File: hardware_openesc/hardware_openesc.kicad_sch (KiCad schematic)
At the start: 0 parts

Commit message: images
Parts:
- added C1, C2: 1u, symbol Device:C_Small
- added Q1, Q2, Q3, Q4, Q5, Q6: BSC007N04LS6, easyeda2kicad:PG-TDSON-8-FL_L5.0-W6.0-P1.27-LS6.2-BL, symbol easyeda2kicad:BSC007N04LS6
- added U1: EFM8BB21F16G-C-QFN20, easyeda2kicad:QFN-20_L3.0-W3.0-P0.50-BL-EP1.7_EFM8BB21F16G, symbol easyeda2kicad:EFM8BB21F16G-C-QFN20
- added U2: FD6288Q_C328453, easyeda2kicad:QFN-24_L4.0-W4.0-P0.50-BL-EP2.6, symbol easyeda2kicad:FD6288Q_C328453
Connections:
- new net: C1.2, C2.2, U1.4 (VDD)
- new net: Q6.1 (S), Q6.2 (S), Q6.3 (S)
- new net: Q5.1 (S), Q5.2 (S), Q5.3 (S), Q6.5 (D), Q6.6 (D), Q6.7 (D), Q6.8 (D)
- new net: Q5.5 (D), Q5.6 (D), Q5.7 (D), Q5.8 (D)
- new net: Q3.1 (S), Q3.2 (S), Q3.3 (S), Q4.5 (D), Q4.6 (D), Q4.7 (D), Q4.8 (D)
- new net: Q3.5 (D), Q3.6 (D), Q3.7 (D), Q3.8 (D)
- new net: Q2.1 (S), Q2.2 (S), Q2.3 (S)
- new net: Q1.1 (S), Q1.2 (S), Q1.3 (S), Q2.5 (D), Q2.6 (D), Q2.7 (D), Q2.8 (D)
- new net: Q4.1 (S), Q4.2 (S), Q4.3 (S)
- new net: Q1.5 (D), Q1.6 (D), Q1.7 (D), Q1.8 (D)
- new net GND: C1.1, C2.1, U1.12 (GND), U1.21 (GND), U1.3 (GND)
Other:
- note added: "A"
- note added: "B"
- note added: "C"

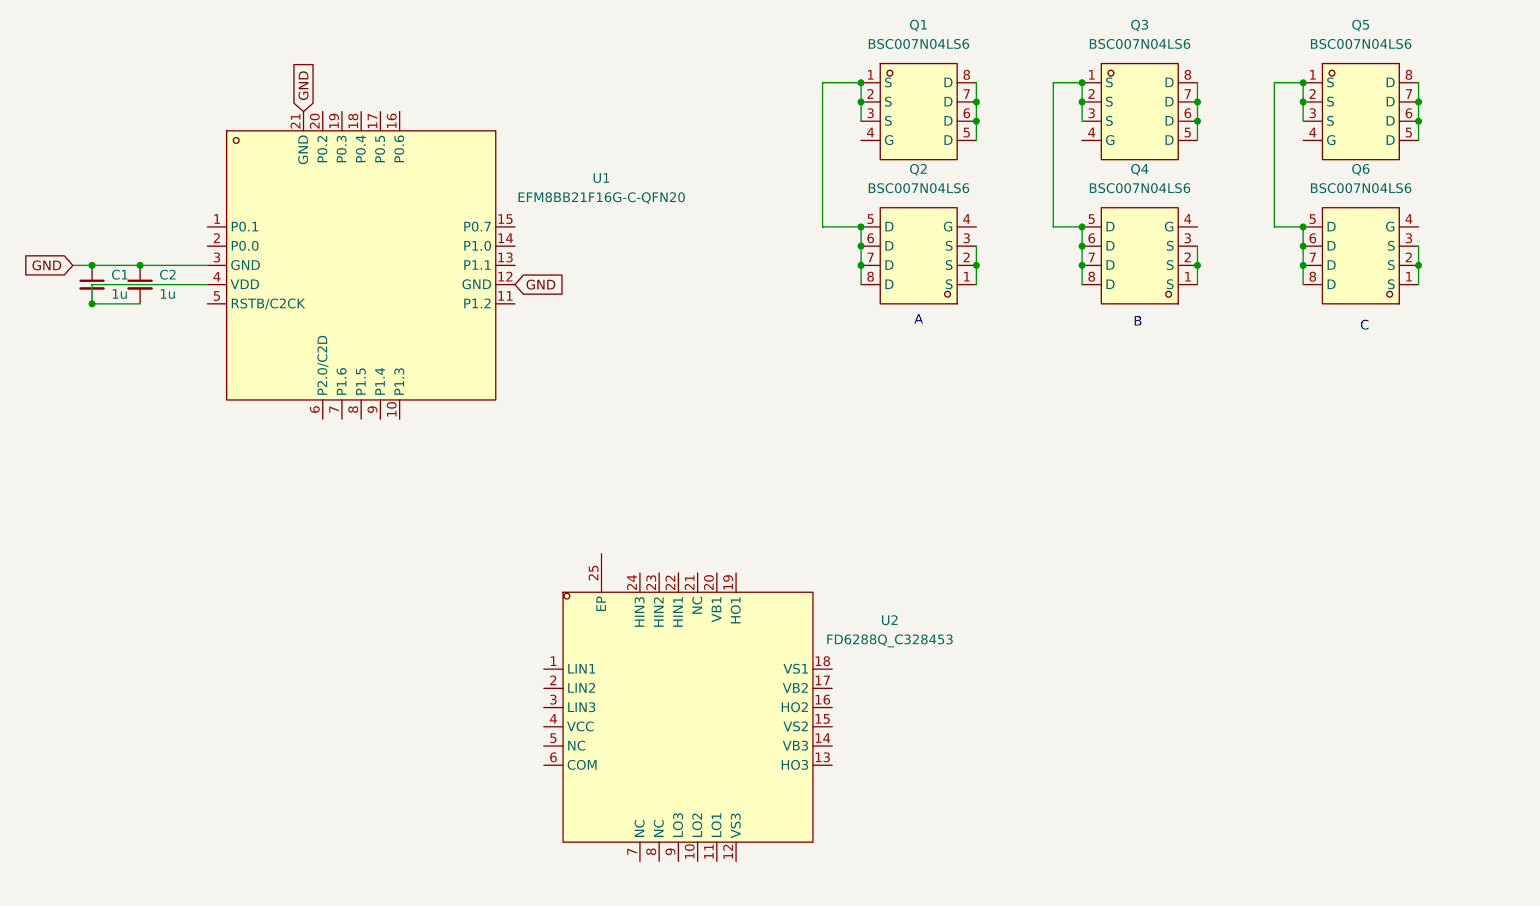
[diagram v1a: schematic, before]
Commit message: schematic
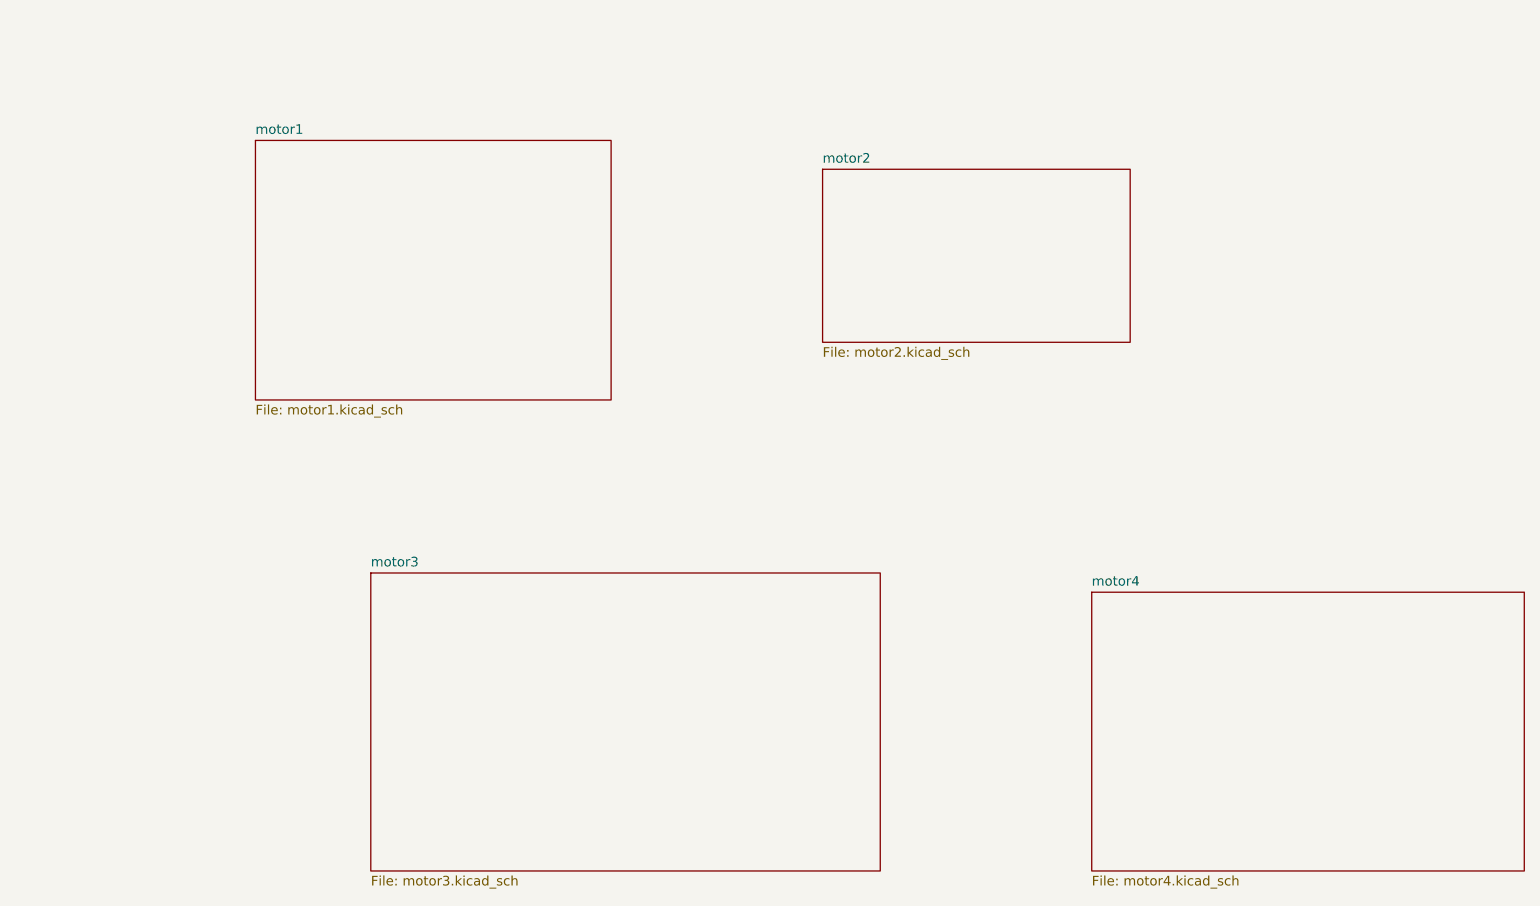
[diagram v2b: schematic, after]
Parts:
- removed C1, C2: 1u, symbol Device:C_Small
- removed Q1, Q2, Q3, Q4, Q5, Q6: BSC007N04LS6, easyeda2kicad:PG-TDSON-8-FL_L5.0-W6.0-P1.27-LS6.2-BL, symbol easyeda2kicad:BSC007N04LS6
- removed U1: EFM8BB21F16G-C-QFN20, easyeda2kicad:QFN-20_L3.0-W3.0-P0.50-BL-EP1.7_EFM8BB21F16G, symbol easyeda2kicad:EFM8BB21F16G-C-QFN20
- removed U2: FD6288Q_C328453, easyeda2kicad:QFN-24_L4.0-W4.0-P0.50-BL-EP2.6, symbol easyeda2kicad:FD6288Q_C328453
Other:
- added sheet motor1 (motor1.kicad_sch)
- added sheet motor2 (motor2.kicad_sch)
- added sheet motor3 (motor3.kicad_sch)
- added sheet motor4 (motor4.kicad_sch)
- note removed: "A"
- note removed: "B"
- note removed: "C"

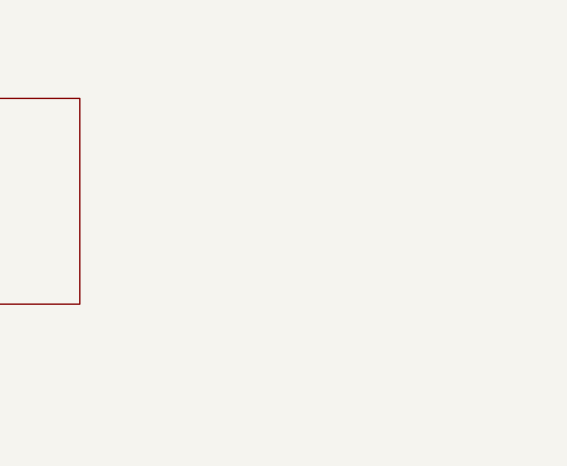
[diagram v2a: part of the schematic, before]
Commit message: schematic
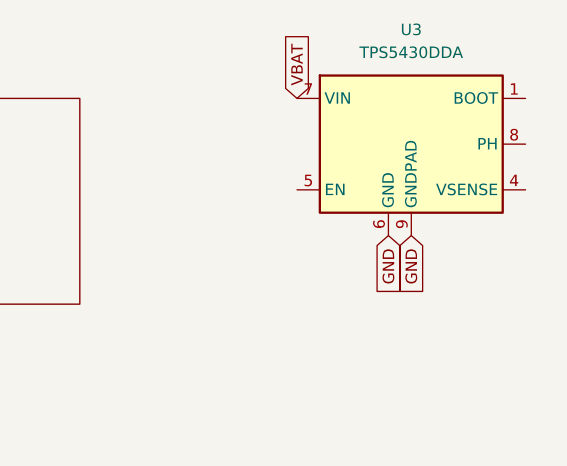
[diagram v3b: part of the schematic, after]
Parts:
- added U3: TPS5430DDA, Package_SO:TI_SO-PowerPAD-8_ThermalVias, symbol Regulator_Switching:TPS5430DDA
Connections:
- new net GND: U3.6 (GND), U3.9 (GNDPAD)
- new net VBAT: U3.7 (VIN)
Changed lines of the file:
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@@
 	(generator_version "9.0")
 	(paper "A4")
+	(global_label "GND"
+		(shape input)
+		(at 199.39 64.77 270)
+		(fields_autoplaced yes)
+		(effects
+			(font
+				(size 1.27 1.27)
+			)
+			(justify right)
+		)
+		(property "Intersheetrefs" "${INTERSHEET_REFS}"
+			(at 199.39 71.6257 90)
+			(effects
+				(font
+					(size 1.27 1.27)
+				)
+				(justify right)
+				(hide yes)
+			)
+		)
+	)
+	(global_label "GND"
+		(shape input)
+		(at 196.85 64.77 270)
+		(fields_autoplaced yes)
+		(effects
+			(font
+				(size 1.27 1.27)
+			)
+			(justify right)
+		)
+		(property "Intersheetrefs" "${INTERSHEET_REFS}"
+			(at 196.85 71.6257 90)
+			(effects
+				(font
+					(size 1.27 1.27)
+				)
+				(justify right)
+				(hide yes)
+			)
+		)
+	)
+	(global_label "VBAT"
+		(shape input)
+		(at 186.69 49.53 90)
+		(fields_autoplaced yes)
+		(effects
+			(font
+				(size 1.27 1.27)
+			)
+			(justify left)
+		)
+		(property "Intersheetrefs" "${INTERSHEET_REFS}"
+			(at 186.69 42.13 90)
+			(effects
+				(font
+					(size 1.27 1.27)
+				)
+				(justify left)
+				(hide yes)
+			)
+		)
+	)
+	(symbol
+		(lib_id "Regulator_Switching:TPS5430DDA")
+		(at 199.39 54.61 0)
+		(unit 1)
+		(exclude_from_sim no)
+		(in_bom yes)
+		(on_board yes)
+		(dnp no)
+		(fields_autoplaced yes)
+		(property "Reference" "U3"
+			(at 199.39 41.91 0)
+			(effects
+				(font
+					(size 1.27 1.27)
+				)
+			)
+		)
+		(property "Value" "TPS5430DDA"
+			(at 199.39 44.45 0)
+			(effects
+				(font
+					(size 1.27 1.27)
+				)
+			)
+		)
+		(property "Footprint" "Package_SO:TI_SO-PowerPAD-8_ThermalVias"
+			(at 200.66 63.5 0)
+			(effects
+				(font
+					(size 1.27 1.27)
+					(italic yes)
+				)
+				(justify left)
+				(hide yes)
+			)
+		)
+		(property "Datasheet" "http://www.ti.com/lit/ds/symlink/tps5430.pdf"
+			(at 199.39 54.61 0)
+			(effects
+				(font
+					(size 1.27 1.27)
+				)
+				(hide yes)
+			)
+		)
+		(property "Description" "3A, Step Down Swift Converter, Adjustable Output Voltage, 5.5-36V Input Voltage, PowerSO-8"
+			(at 199.39 54.61 0)
+			(effects
+				(font
+					(size 1.27 1.27)
+				)
+				(hide yes)
+			)
+		)
+		(pin "2"
+		)
+		(pin "8"
+		)
+		(pin "7"
+		)
+		(pin "5"
+		)
+		(pin "6"
+		)
+		(pin "1"
+		)
+		(pin "9"
+		)
+		(pin "3"
+		)
+		(pin "4"
+		)
+		(instances
+			(project "hardware_openesc"
+				(path "/fd04cde8-8623-46f8-9b2f-1ba4eb308030"
+					(reference "U3")
+					(unit 1)
+				)
+			)
+		)
+	)
 	(sheet
 		(at 62.23 102.87)
